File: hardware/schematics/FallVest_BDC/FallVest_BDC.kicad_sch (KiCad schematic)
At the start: 10 parts, among them IC1 ATGM336H-5N31, J1 Actuator, J2 MG90S_SERVO, Q1 AO3400A, U1 SIM800L-CORE, U2 ESP32-WROOM-32, U3 MPU-6050

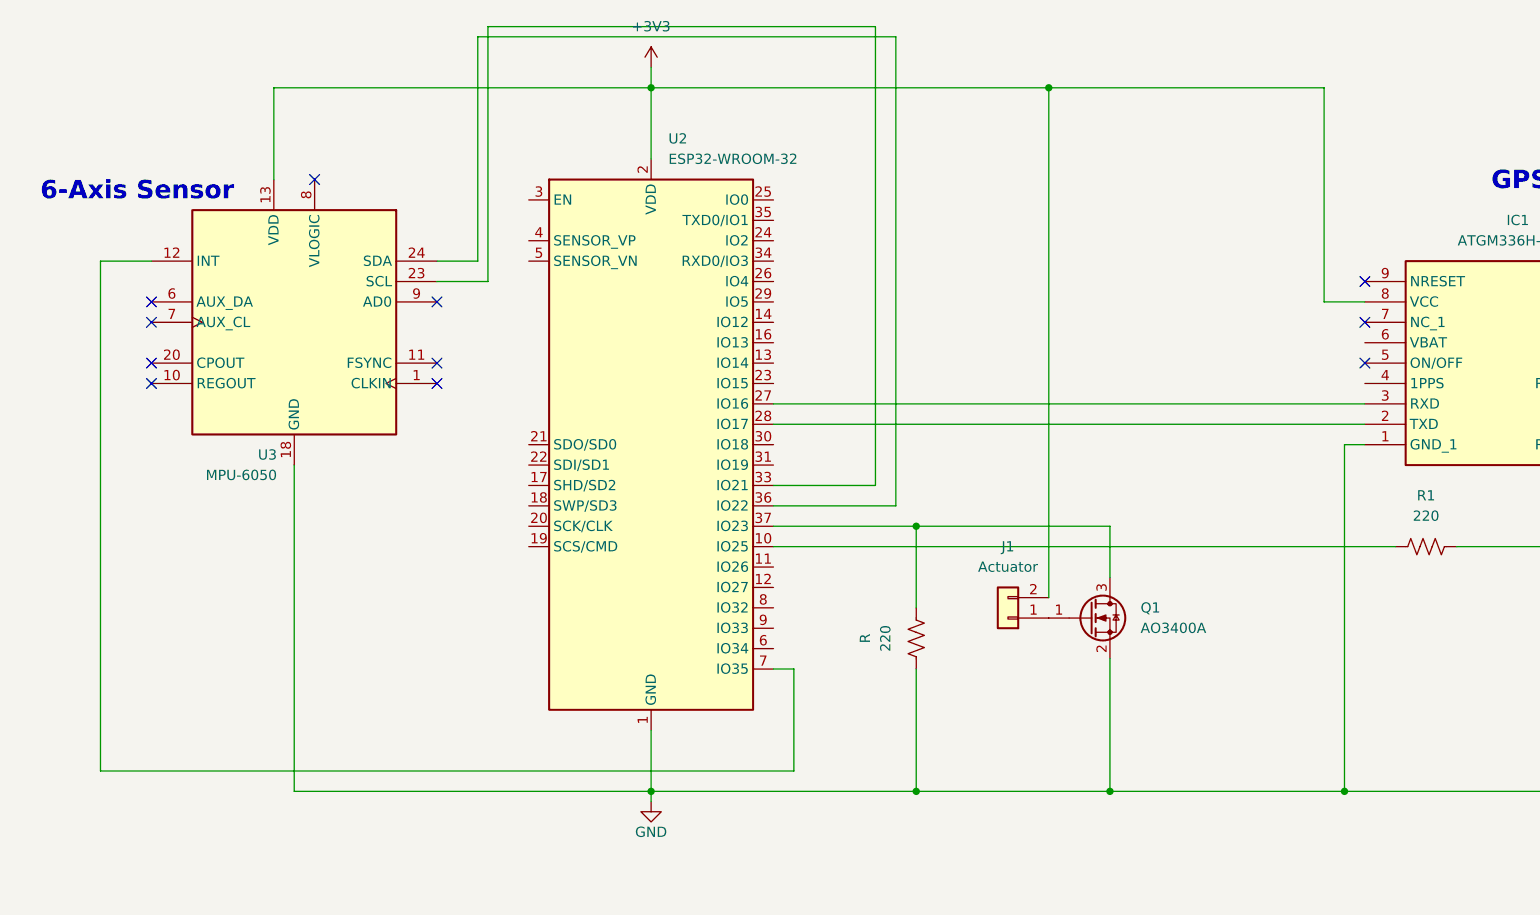
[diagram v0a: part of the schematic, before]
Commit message: Replaced bare module
- Development board ELEGOO
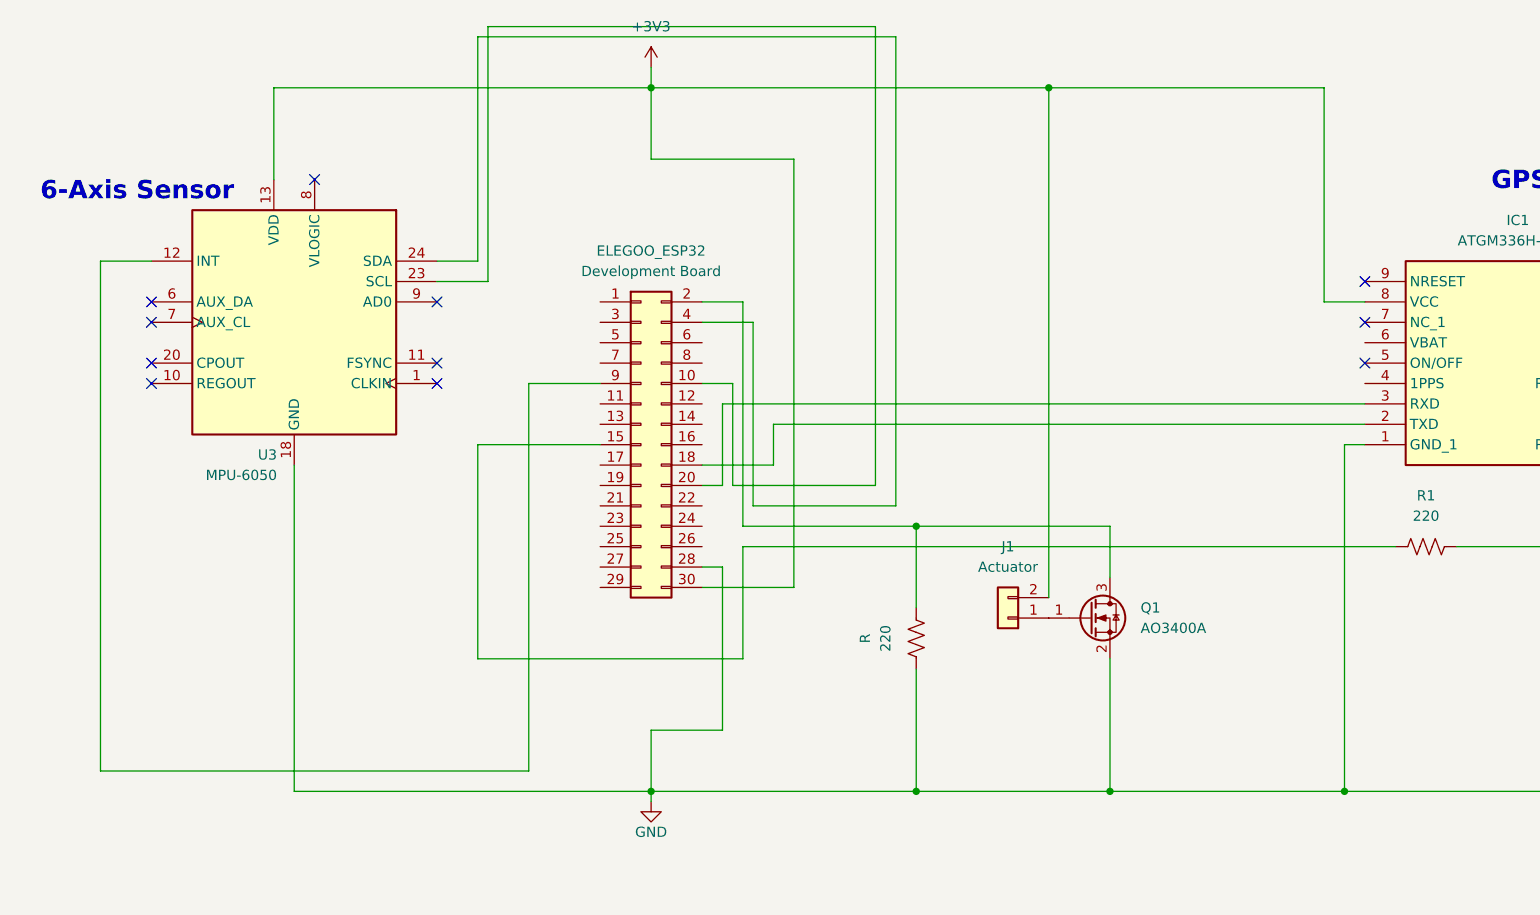
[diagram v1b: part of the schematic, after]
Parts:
- removed U2: ESP32-WROOM-32, RF_Module:ESP32-WROOM-32, symbol RF_Module:ESP32-WROOM-32
- added ELEGOO_ESP32: Development Board, symbol Connector_Generic:Conn_02x15_Odd_Even
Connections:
- net +3V3: now also ELEGOO_ESP32.30 (Pin_30)
- net GND: now also ELEGOO_ESP32.28 (Pin_28)
- net at Q1.3 (D), R.2: now also ELEGOO_ESP32.2 (Pin_2)
- net at IC1.2 (TXD): now also ELEGOO_ESP32.18 (Pin_18)
- net at IC1.3 (RXD): now also ELEGOO_ESP32.20 (Pin_20)
- net at U3.12 (INT): now also ELEGOO_ESP32.9 (Pin_9)
- net at U3.23 (SCL): now also ELEGOO_ESP32.10 (Pin_10)
- net at U3.24 (SDA): now also ELEGOO_ESP32.4 (Pin_4)
- net at R1.2: now also ELEGOO_ESP32.15 (Pin_15)
